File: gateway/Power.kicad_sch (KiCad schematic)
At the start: 58 parts, among them IC701 LM62460, IC702 ADP1614ACPZ-R7, IC703 TPS2121RUXT, IC704 MIC5317-1.8xM5, IC705 MIC5317-3.3xM5, X701 7-24 V

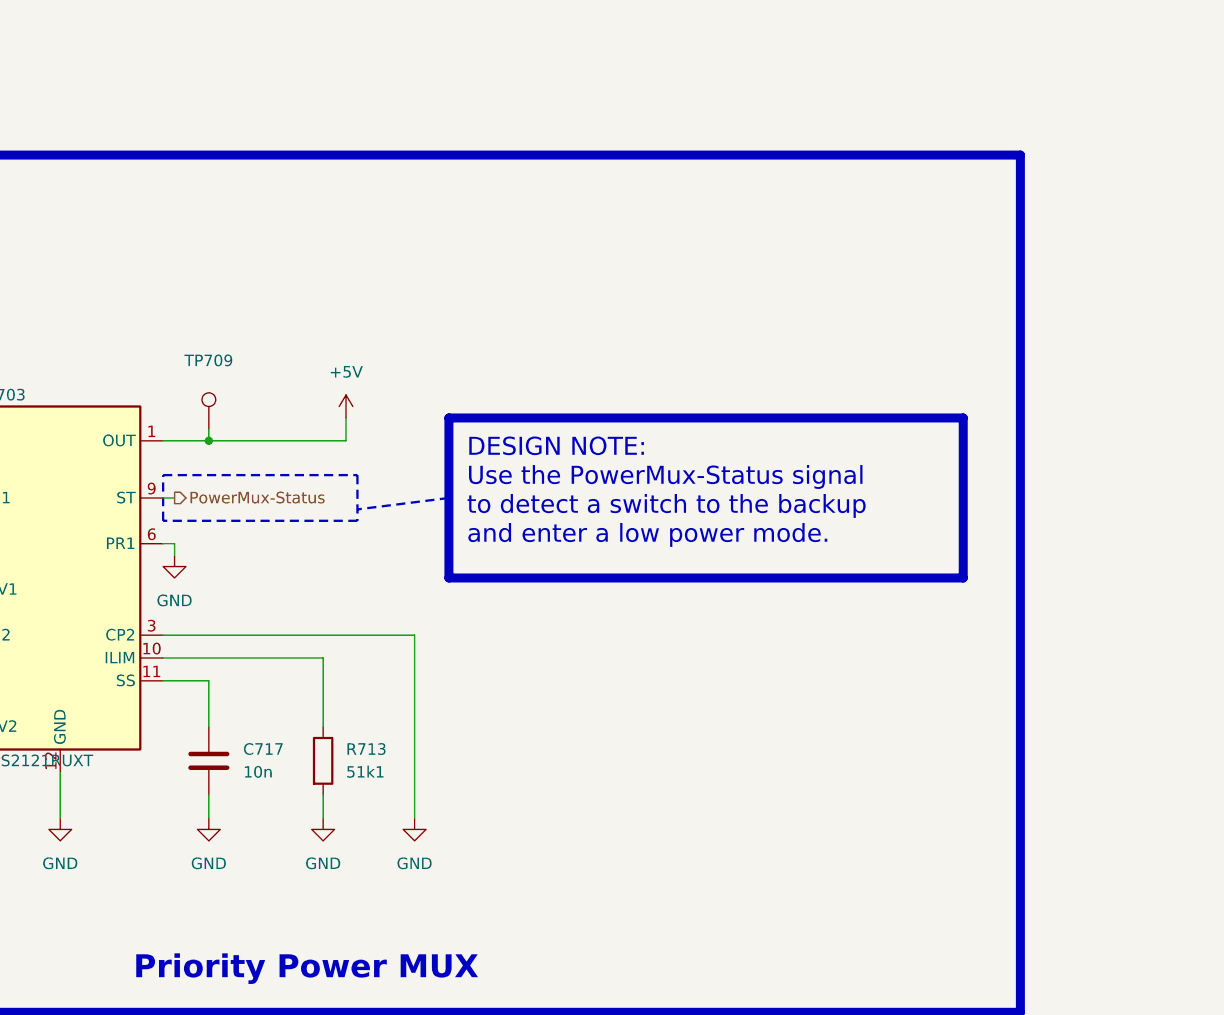
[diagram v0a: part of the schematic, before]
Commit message: Working on first version
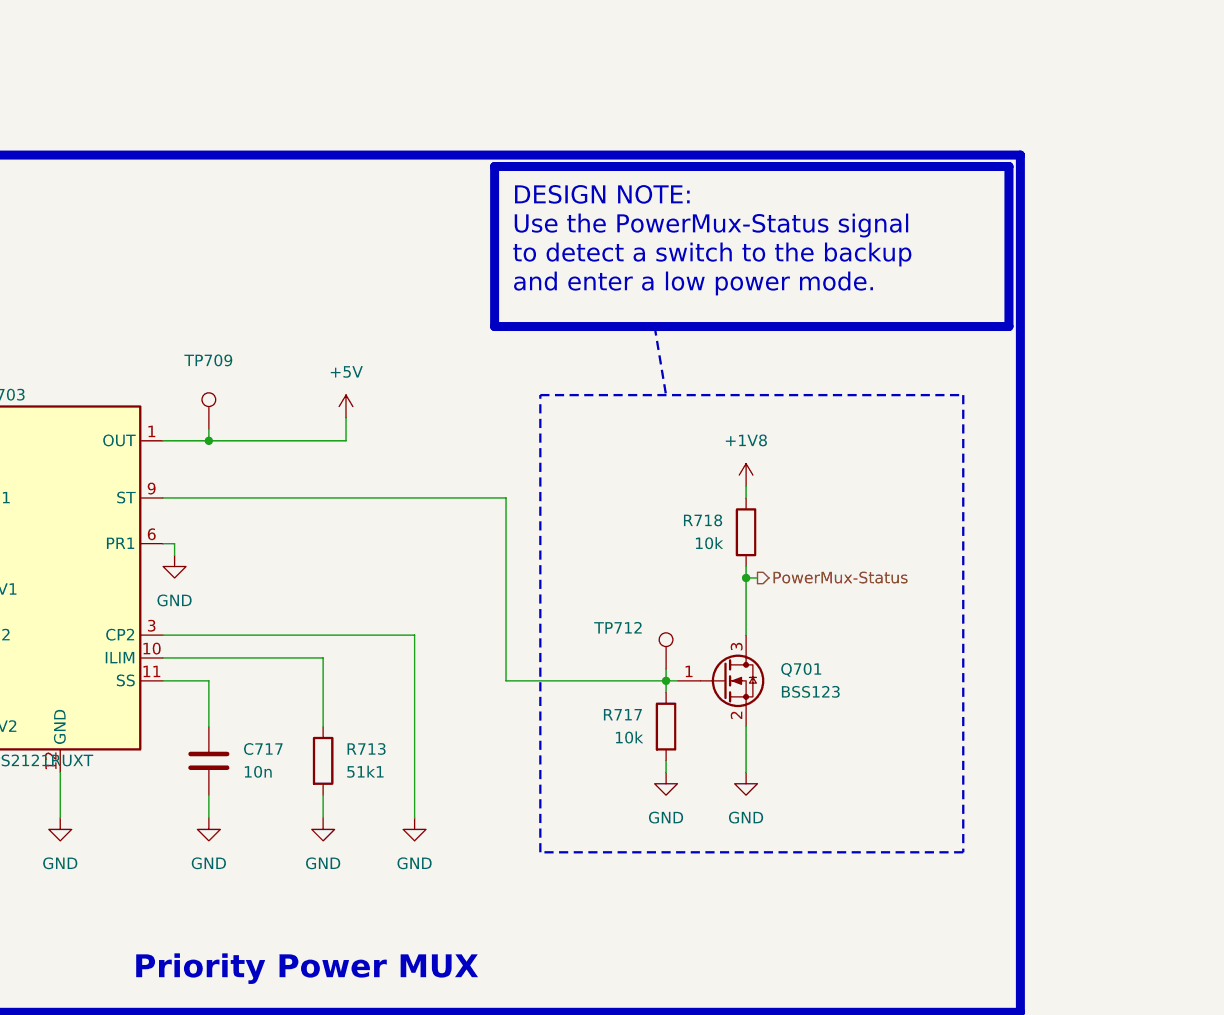
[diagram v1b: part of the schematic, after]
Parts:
- added Q701: BSS123, Package_TO_SOT_SMD:SOT-23, symbol Transistor_FET:BSS123
- added R717, R718: 10k, symbol Device:R
- added TP712: ~, symbol Connector:TestPoint
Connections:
- net +1V8: now also R718.1
- net GND: now also Q701.2 (S), R717.2
- net PowerMux-Status: now also Q701.3 (D), R718.2; no longer IC703.9 (ST)
- new net: IC703.9 (ST), Q701.1 (G), R717.1, TP712.1

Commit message: Working on version 1.0
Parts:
- C703: footprint (none) -> Capacitor_SMD:C_0805_2012Metric; manf (none) -> KYOCERA AVX; manf# (none) -> 08056C105MAT2A; mouser# (none) -> 581-08056C105MAT2A
- C704: footprint Capacitor_SMD:C_0402_1005Metric -> Capacitor_SMD:C_0805_2012Metric; manf# 04023C473KAT4A -> 08053C473K4T2A; mouser# 581-04023C473KAT4A -> 581-08053C473K4T2A
- C705, C706: footprint (none) -> Capacitor_SMD:C_0805_2012Metric; manf (none) -> KYOCERA AVX; manf# (none) -> 08053C474K4T4A; mouser# (none) -> 581-08053C474K4T4A
- C708: footprint Capacitor_SMD:C_0402_1005Metric -> Capacitor_SMD:C_0805_2012Metric; manf# 04025C104JAT2A -> 08053C104M4T4A; mouser# (none) -> 581-08053C104M4T4A
- C709, C711, C713, C714, C715: footprint (none) -> Capacitor_SMD:C_0805_2012Metric; manf (none) -> KYOCERA AVX; manf# (none) -> KGM21AR51A226MU; mouser# (none) -> 581-KGM21AR51A226MU
- C710: footprint Capacitor_SMD:C_0402_1005Metric -> Capacitor_SMD:C_0805_2012Metric; manf# 04023C223KAT2A -> 08052C223M4Z2A; mouser# 581-04023C223KAT2A -> 581-08052C223M4Z2A
- C712: footprint Capacitor_SMD:C_0402_1005Metric -> Capacitor_SMD:C_0805_2012Metric; manf# 04021A330JAT2A -> 08053C330KAT2A; mouser# 581-04021A330JAT2A -> 581-08053C330KAT2A
- C716: footprint (none) -> Capacitor_SMD:C_0805_2012Metric; manf (none) -> KYOCERA AVX; manf# (none) -> 08053A100JAT2A; mouser# (none) -> 581-08053A100JAT2A
- C717: renamed from C720; footprint (none) -> Capacitor_SMD:C_0805_2012Metric; manf (none) -> KYOCERA AVX; manf# (none) -> 08056C105MAT2A; mouser# (none) -> 581-08056C105MAT2A
- C718: renamed from C717; footprint Capacitor_SMD:C_0402_1005Metric -> Capacitor_SMD:C_0805_2012Metric; manf# 0402X7R103KT2AT -> 08055C103K4T4A; mouser# 581-0402X7R103KT2AT -> 581-08055C103K4T4A
- C719: renamed from C721; footprint (none) -> Capacitor_SMD:C_0805_2012Metric; manf (none) -> KYOCERA AVX; manf# (none) -> 08056C105MAT2A; mouser# (none) -> 581-08056C105MAT2A
- C720: renamed from C718; footprint (none) -> Capacitor_SMD:C_0805_2012Metric; manf (none) -> KYOCERA AVX; manf# (none) -> 08056C105MAT2A; mouser# (none) -> 581-08056C105MAT2A; now left out of the parts list
- C721: renamed from C719; footprint (none) -> Capacitor_SMD:C_0805_2012Metric; manf (none) -> KYOCERA AVX; manf# (none) -> 08056C105MAT2A; mouser# (none) -> 581-08056C105MAT2A; now left out of the parts list
- IC701: manf (none) -> Texas Instruments; manf# (none) -> LM62460; mouser# (none) -> 595-LM62460
- IC704: renamed from IC705; manf (none) -> Microchip Technology; manf# (none) -> MIC5317-3.3YM5-TR; mouser# (none) -> 998-MIC5317-3.3YM5-TR
- IC705: renamed from IC704; manf (none) -> Microchip Technology; manf# (none) -> MIC5317-1.8YM5-TR; mouser# (none) -> 998-MIC5317-1.8YM5-TR; now left out of the parts list
- L702: value 2u7 -> 2u2; footprint (none) -> Inductor_SMD:L_Wuerth_WE-PD-Typ-7345; manf (none) -> Wurth Elektronik; manf# (none) -> 744777002; mouser# (none) -> 710-744777002
- R701: footprint (none) -> Resistor_SMD:R_0805_2012Metric; manf (none) -> Bourns; manf# (none) -> CR0805-JW-103GLF; mouser# (none) -> 652-CR0805-JW-103GLF
- R703: footprint Resistor_SMD:R_0402_1005Metric -> Resistor_SMD:R_0805_2012Metric; manf# CR0402-JW-202GLF -> CR0805-JW-202GLF; mouser# 652-CR0402-JW-202GLF -> 652-CR0805-JW-202GLF
- R704: footprint Resistor_SMD:R_0402_1005Metric -> Resistor_SMD:R_0805_2012Metric; manf# CR0402-FX-3092GLF -> CR0805-FX-3092GLF; mouser# 652-CR0402-FX-3092GLF -> 652-CR0805-FX-3092GLF
- R705: footprint Resistor_SMD:R_0402_1005Metric -> Resistor_SMD:R_0805_2012Metric; manf# CR0402-JW-103GLF -> CR0805-JW-103GLF; mouser# 652-CR0402-JW-103GLF -> 652-CR0805-JW-103GLF
- R706: footprint Resistor_SMD:R_0402_1005Metric -> Resistor_SMD:R_0805_2012Metric; manf# CR0402-JW-104GLF -> CR0805-JW-104GLF; mouser# 652-CR0402-JW-104GLF -> 652-CR0805-JW-104GLF
- R707: footprint (none) -> Resistor_SMD:R_0805_2012Metric; manf (none) -> Bourns; manf# (none) -> CR0805-FX-2492ELF; mouser# (none) -> 652-CR0805-FX-2492ELF
- R708: footprint (none) -> Resistor_SMD:R_0805_2012Metric; manf (none) -> Bourns; manf# (none) -> CR0805-FX-4991ELF; mouser# (none) -> 652-CR0805-FX-4991ELF
- R709, R711: footprint Resistor_SMD:R_0402_1005Metric -> Resistor_SMD:R_0805_2012Metric; manf# CR0402-FX-2102GLF -> CR0805-FX-2102GLF; mouser# 652-CR0402-FX-2102GLF -> 652-CR0805-FX-2102GLF
- R710, R712: footprint Resistor_SMD:R_0402_1005Metric -> Resistor_SMD:R_0805_2012Metric; manf# CR0402-JW-512GLF -> CR0805-JW-512GLF; mouser# 652-CR0402-JW-512GLF -> 652-CR0805-JW-512GLF
- R713: renamed from R716; footprint (none) -> Resistor_SMD:R_0805_2012Metric; manf (none) -> Bourns; manf# (none) -> CR0805-JW-103GLF; mouser# (none) -> 652-CR0805-JW-103GLF
- R714: renamed from R713; footprint Resistor_SMD:R_0402_1005Metric -> Resistor_SMD:R_0805_2012Metric; manf# CR0402-FX-5112GLF -> CR0805-FX-5112GLF; mouser# 652-CR0402-FX-5112GLF -> 652-CR0805-FX-5112GLF
- R715: renamed from R717; footprint (none) -> Resistor_SMD:R_0805_2012Metric; manf (none) -> Bourns; manf# (none) -> CR0805-JW-103GLF; mouser# (none) -> 652-CR0805-JW-103GLF
- R716: renamed from R718; footprint (none) -> Resistor_SMD:R_0805_2012Metric; manf (none) -> Bourns; manf# (none) -> CR0805-JW-103GLF; mouser# (none) -> 652-CR0805-JW-103GLF
- R717: renamed from R714; footprint (none) -> Resistor_SMD:R_0805_2012Metric; manf (none) -> Bourns; manf# (none) -> CR0805-FX-1002GLF; mouser# (none) -> 652-CR0805-FX-1002GLF; now left out of the parts list
- TP701, TP706: footprint (none) -> Testpoints_Kampi:TestPoint_Pad_1.0x1.0mm; now left out of the parts list
- TP703, TP704: footprint (none) -> Testpoints_Kampi:TestPoint_Pad_1.0x1.0mm
- TP710: renamed from TP711; footprint (none) -> Testpoints_Kampi:TestPoint_Pad_1.0x1.0mm
- TP711: renamed from TP712; footprint (none) -> Testpoints_Kampi:TestPoint_Pad_1.0x1.0mm
- TP712: renamed from TP710; footprint (none) -> Testpoints_Kampi:TestPoint_Pad_1.0x1.0mm
- X701: value 7-24 V -> 7-16 V; footprint (none) -> Connector_BarrelJack:BarrelJack_Wuerth_6941xx301002; symbol Connector_Generic:Conn_01x02 -> Connector:Barrel_Jack; manf (none) -> Wurth Elektronik; manf# (none) -> 694102303002; mouser# (none) -> 710-694102303002
- renumbered R715 to R718
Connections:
- net GND: now also X701.2; no longer X701.1 (Pin_1)
- net at F701.1: now also X701.1; no longer X701.2 (Pin_2)
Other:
- moved on the sheet: C701, C702, C703, C705, C706, C707, C708, C709, C711, C713, C714, C715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
